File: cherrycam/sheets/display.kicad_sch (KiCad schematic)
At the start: 2 parts, among them J4 Conn_01x08, Q1 BSS138

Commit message: footprints + pcb + new journal
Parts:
- J4: footprint (none) -> Connector_PinHeader_2.54mm:PinHeader_1x08_P2.54mm_Vertical
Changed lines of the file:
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@@
 			)
 		)
-		(property "Footprint" ""
+		(property "Footprint" "Connector_PinHeader_2.54mm:PinHeader_1x08_P2.54mm_Vertical"
 			(at 179.07 91.44 0)
 			(hide yes)

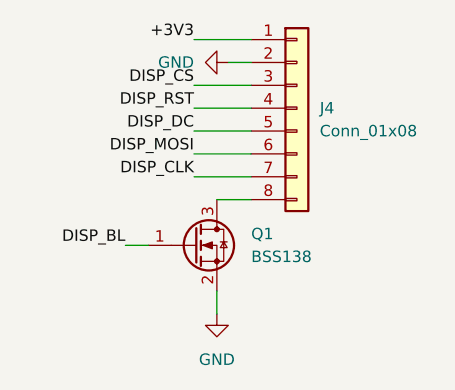
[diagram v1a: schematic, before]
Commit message: new update
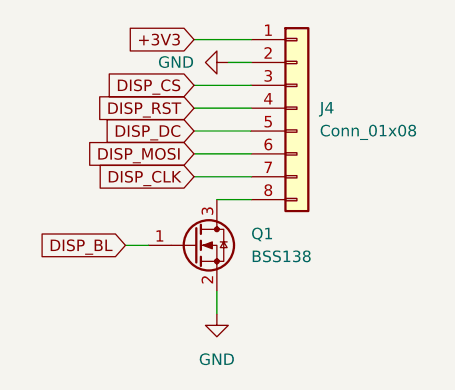
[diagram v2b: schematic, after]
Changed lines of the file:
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@@
 		)
 	)
-	(label "DISP_MOSI"
-		(at 167.64 96.52 180)
+	(global_label "DISP_RST"
+		(shape input)
+		(at 167.64 91.44 180)
+		(fields_autoplaced yes)
 		(effects
 			(font
 				(size 1.27 1.27)
 			)
-			(justify right bottom)
+			(justify right)
+		)
+		(property "Intersheetrefs" "${INTERSHEET_REFS}"
+			(at 155.8858 91.44 0)
+			(hide yes)
+			(show_name no)
+			(do_not_autoplace no)
+			(effects
+				(font
+					(size 1.27 1.27)
+				)
+				(justify right)
+			)
 		)
 	)
-	(label "+3V3"
-		(at 167.64 83.82 180)
+	(global_label "DISP_BL"
+		(shape input)
+		(at 160.02 106.68 180)
+		(fields_autoplaced yes)
 		(effects
 			(font
 				(size 1.27 1.27)
 			)
-			(justify right bottom)
+			(justify right)
+		)
+		(property "Intersheetrefs" "${INTERSHEET_REFS}"
+			(at 149.4148 106.68 0)
+			(hide yes)
+			(show_name no)
+			(do_not_autoplace no)
+			(effects
+				(font
+					(size 1.27 1.27)
+				)
+				(justify right)
+			)
 		)
 	)
-	(label "DISP_RST"
-		(at 167.64 91.44 180)
+	(global_label "DISP_MOSI"
+		(shape input)
+		(at 167.64 96.52 180)
+		(fields_autoplaced yes)
 		(effects
 			(font
 				(size 1.27 1.27)
 			)
-			(justify right bottom)
+			(justify right)
+		)
+		(property "Intersheetrefs" "${INTERSHEET_REFS}"
+			(at 154.7367 96.52 0)
+			(hide yes)
+			(show_name no)
+			(do_not_autoplace no)
+			(effects
+				(font
+					(size 1.27 1.27)
+				)
+				(justify right)
+			)
 		)
 	)
-	(label "DISP_BL"
-		(at 160.02 106.68 180)
+	(global_label "DISP_DC"
+		(shape input)
+		(at 167.64 93.98 180)
+		(fields_autoplaced yes)
 		(effects
 			(font
 				(size 1.27 1.27)
 			)
-			(justify right bottom)
+			(justify right)
+		)
+		(property "Intersheetrefs" "${INTERSHEET_REFS}"
+			(at 156.7929 93.98 0)
+			(hide yes)
+			(show_name no)
+			(do_not_autoplace no)
+			(effects
+				(font
+					(size 1.27 1.27)
+				)
+				(justify right)
+			)
 		)
 	)
-	(label "DISP_CS"
-		(at 167.64 88.9 180)
+	(global_label "DISP_CLK"
+		(shape input)
+		(at 167.64 99.06 180)
+		(fields_autoplaced yes)
 		(effects
 			(font
 				(size 1.27 1.27)
 			)
-			(justify right bottom)
+			(justify right)
+		)
+		(property "Intersheetrefs" "${INTERSHEET_REFS}"
+			(at 155.7648 99.06 0)
+			(hide yes)
+			(show_name no)
+			(do_not_autoplace no)
+			(effects
+				(font
+					(size 1.27 1.27)
+				)
+				(justify right)
+			)
 		)
 	)
-	(label "DISP_DC"
-		(at 167.64 93.98 180)
+	(global_label "DISP_CS"
+		(shape input)
+		(at 167.64 88.9 180)
+		(fields_autoplaced yes)
 		(effects
 			(font
 				(size 1.27 1.27)
 			)
-			(justify right bottom)
+			(justify right)
+		)
+		(property "Intersheetrefs" "${INTERSHEET_REFS}"
+			(at 156.8534 88.9 0)
+			(hide yes)
+			(show_name no)
+			(do_not_autoplace no)
+			(effects
+				(font
+					(size 1.27 1.27)
+				)
+				(justify right)
+			)
 		)
 	)
-	(label "DISP_CLK"
-		(at 167.64 99.06 180)
+	(global_label "+3V3"
+		(shape input)
+		(at 167.64 83.82 180)
+		(fields_autoplaced yes)
 		(effects
 			(font
 				(size 1.27 1.27)
 			)
-			(justify right bottom)
+			(justify right)
+		)
+		(property "Intersheetrefs" "${INTERSHEET_REFS}"
+			(at 159.5748 83.82 0)
+			(hide yes)
+			(show_name no)
+			(do_not_autoplace no)
+			(effects
+				(font
+					(size 1.27 1.27)
+				)
+				(justify right)
+			)
 		)
 	)
